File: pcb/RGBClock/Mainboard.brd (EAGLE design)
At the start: 99.8 x 70.1 mm, 112 parts, among them IC1 MCP23017SO, K1 G6K-2F, K2 G6K-2F, K3 G6K-2F, K4 G6K-2F, Q1 32.768KHz, U1 MAX6369KA+T, U10 NX3L1G384GW, U11 NX3L1G384GW, U13 DRV612PW, U14 2N7002-7-F, U15 2N7002-7-F, U16 2N7002-7-F, U17 2N7002-7-F, U2 TXS0102DCUR, U3 P82B96DR, U4 LM2675M-5.0, U5 DS1338Z-33+, U8 NX3L1G384GW, U9 NX3L1G384GW, X2 43045-0400, X5 43045-0800, X6 ST-SMB-H

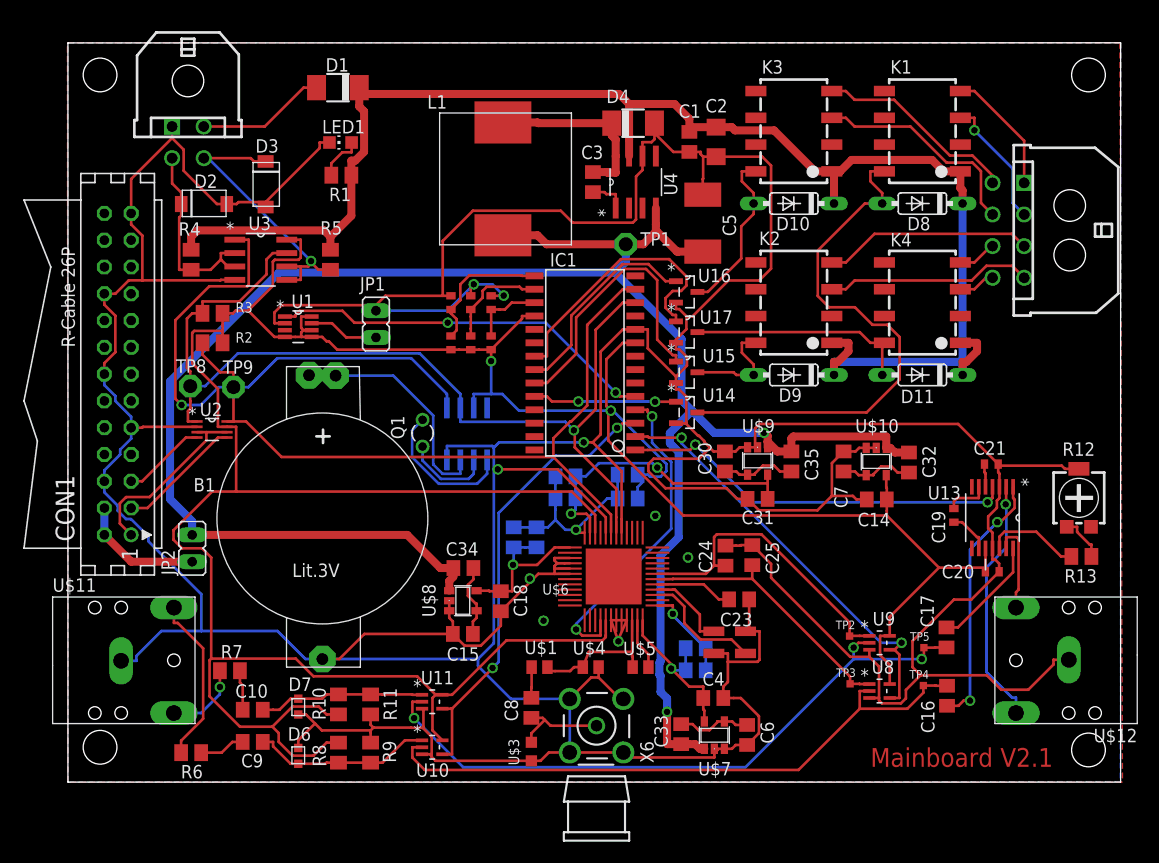
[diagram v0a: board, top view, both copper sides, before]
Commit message: as send to Jclpcb (ver 1.3)
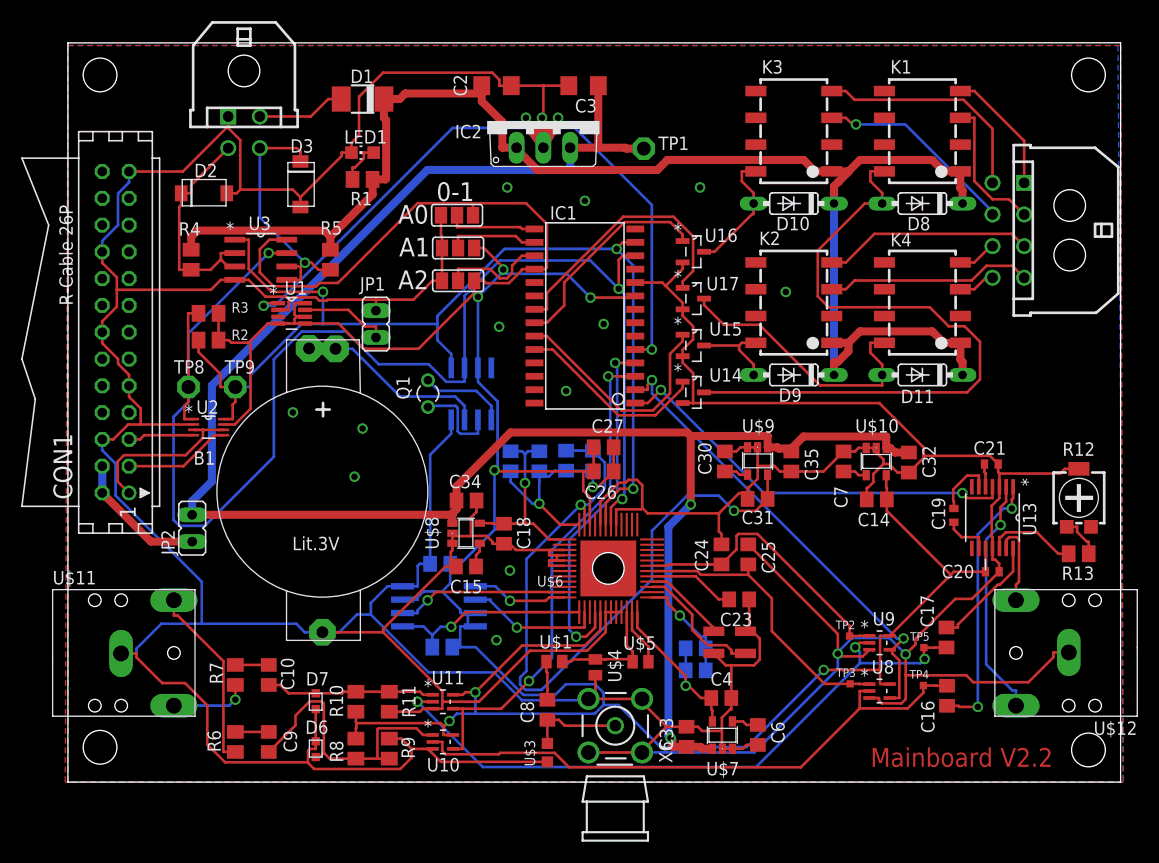
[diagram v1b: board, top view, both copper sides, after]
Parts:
- removed C1: 100n, Mainboard:RCL_C0805
- removed C5: 594D686X0010C2T, Mainboard:MYCOMPONENTS_594D-B
- removed D4: B130-13-F, Mainboard:DIODE_DO-214AC
- removed L1: SRR1240-680M, Mainboard:BOURNS_BY_ELEMENT14_BATCH_1_SRR1240
- removed R14: A2-1, Mainboard:RESISTOR_R0402:1
- removed R15: A2-0, Mainboard:RESISTOR_R0402:1
- removed R16: A1-1, Mainboard:RESISTOR_R0402:1
- removed R17: A1-0, Mainboard:RESISTOR_R0402:1
- removed R18: A0-1, Mainboard:RESISTOR_R0402:1
- removed R19: A0-0, Mainboard:RESISTOR_R0402:1
- removed U4: LM2675M-5.0, Mainboard:TEXAS_SOIC127P620X175-8N
- added C36: 100n, Mainboard:RCL_C0805
- added IC2: R-78B5.0-2.0, linear:TO220V
- added R20: 3K48, rcl:M0805
- added SJ1: A2, jumper:SJ_2
- added SJ2: A1, jumper:SJ_2
- added SJ3: A0, jumper:SJ_2
- added U$13: SST26VF032B, Mainboard:SOIJ8
- C2: value 4,7u -> 10u
- C3: value 10n -> 10u; device Mainboard:RCL_C0805 -> Mainboard:RCL_C1206
- CON1: device Mainboard:CON-HARTING_CON26 -> con-harting:CON26
- moved C2 21.5 mm to (40.6, 66.0), turned to 0 degrees
- moved TP1 9.23 mm to (54.6, 60.1)
- moved C3 9.19 mm to (48.9, 66.0), turned to 180 degrees
- moved C28 7.23 mm to (42.0, 30.4), turned to 90 degrees
- moved C29 7.23 mm to (44.7, 30.4), turned to 90 degrees
- moved C18 6.41 mm to (41.4, 23.6)
- moved U$8 6.41 mm to (37.8, 23.6)
- moved C15 6.41 mm to (37.8, 20.4)
- moved C34 6.41 mm to (37.8, 26.7)
- moved X2 5.40 mm to (16.7, 67.4)
- moved IC1 4.45 mm to (49.0, 43.6)
- moved R6 4.31 mm to (15.9, 3.81), turned to 270 degrees
- moved CON1 3.98 mm to (4.53, 42.7)
- moved U16 3.86 mm to (59.3, 50.3)
- moved U5 3.82 mm to (38.2, 36.8)
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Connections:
- removed net N$42: IC1.16, R16.1, R17.2
- removed net N$43: IC1.17, R14.1, R15.2
- new net N$71: U$13.6, U$6.2
- new net N$72: U$13.2, U$6.47
- new net N$73: R20.2, U$13.1, U$6.1
- new net N$74: U$13.5, U$6.48
- net +3V3: now also C36.1, R20.1, SJ1.1, SJ2.1, SJ3.1, U$13.3, U$13.7, U$13.8; no longer R14.2, R16.2, R18.2
- net +5V: now also C3.1, IC2.3; no longer C5.P$1, L1.1, U4.4
- net GND: now also C3.2, C32.2, C33.2, C34.2, C35.2, C36.2, IC2.2, SJ1.3, SJ2.3, SJ3.3, U$13.4; no longer C1.2, C5.P$2, D4.A, R15.1, R17.1, R19.1, U4.6
- net N$10: now also IC1.17, SJ1.2; no longer C3.1, U4.1
- net N$11: now also IC1.16, SJ2.2; no longer C3.2, D4.C, L1.2, U4.8
- net N$39: no longer C33.2
- net N$41: now also SJ3.2; no longer R18.1, R19.2
- net N$58: no longer C34.2
- net N$62: no longer C35.2
- net N$65: no longer C32.2
- net VCC: now also IC2.1; no longer C1.1, U4.7
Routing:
- net SCL: track 93.2 -> 138.7 mm, vias 1 -> 3
- net +1.8-MEM: track 28.9 -> 68.4 mm
- net N$33: track 36.9 -> 63.6 mm
- net SDA: track 123.0 -> 103.9 mm, vias 1 -> 3
- net N$73: track 0.00 -> 19.1 mm, vias 0 -> 1
- net N$72: track 0.00 -> 16.3 mm, vias 0 -> 1
- net +5V: track 195.5 -> 181.5 mm
- net N$22: track 51.0 -> 64.6 mm
- net N$71: track 0.00 -> 13.0 mm, vias 0 -> 1
- net GND: track 633.9 -> 645.9 mm, vias 9 -> 17
- net N$37: track 17.1 -> 28.2 mm
- net N$42: track 9.92 -> 0.00 mm
- net N$74: track 0.00 -> 9.16 mm, vias 0 -> 1
- net N$11: track 17.4 -> 8.62 mm
- net VCC: track 145.5 -> 137.6 mm
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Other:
- board text added: "0-1"
- board text added: "A0"
- board text added: "A1"
- board text added: "A2"
- board text added: "Mainboard V2.2"
- board text removed: "Mainboard V2.1"
